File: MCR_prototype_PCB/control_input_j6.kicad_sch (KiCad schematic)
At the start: 34 parts, among them J6 Conn_01x10_Pin, U4 74AHC165

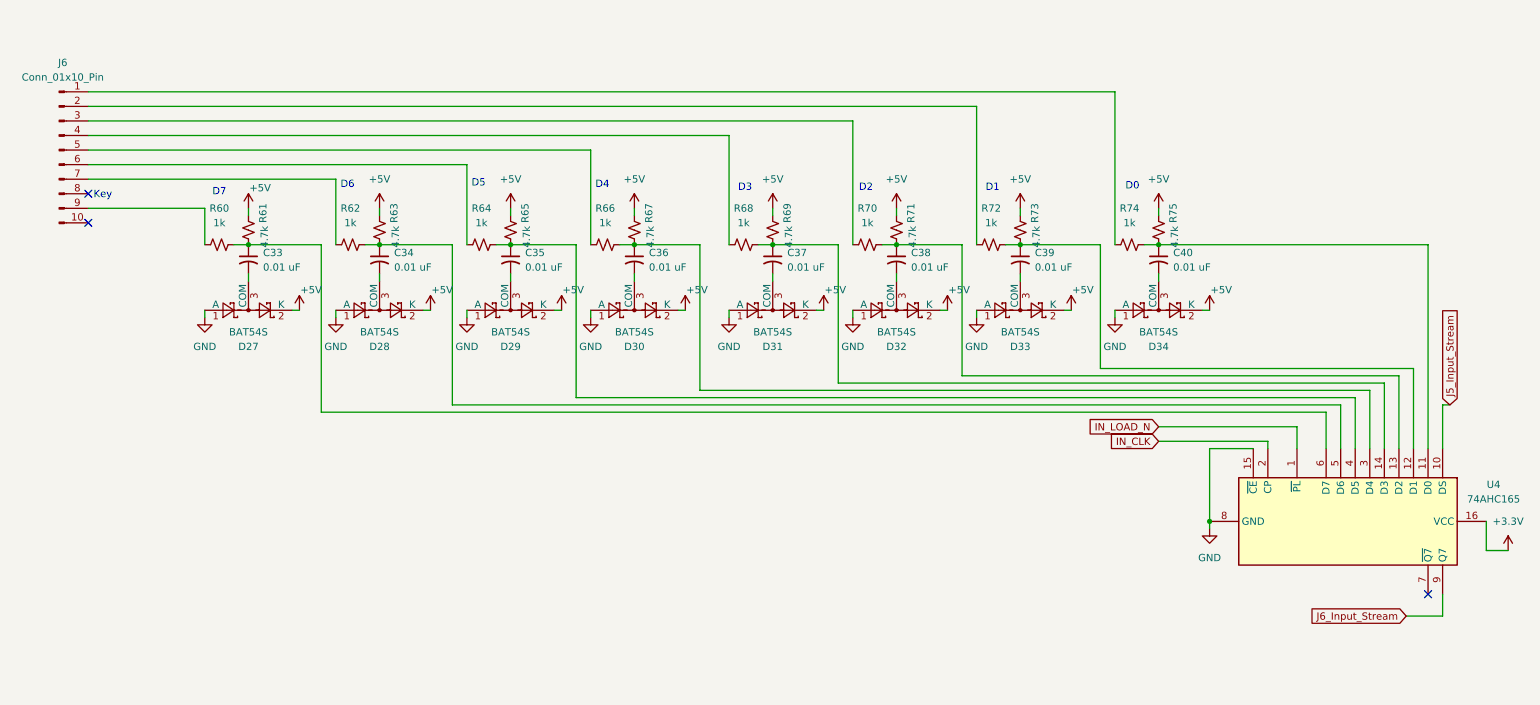
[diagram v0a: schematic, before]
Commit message: Updated 8/22/26
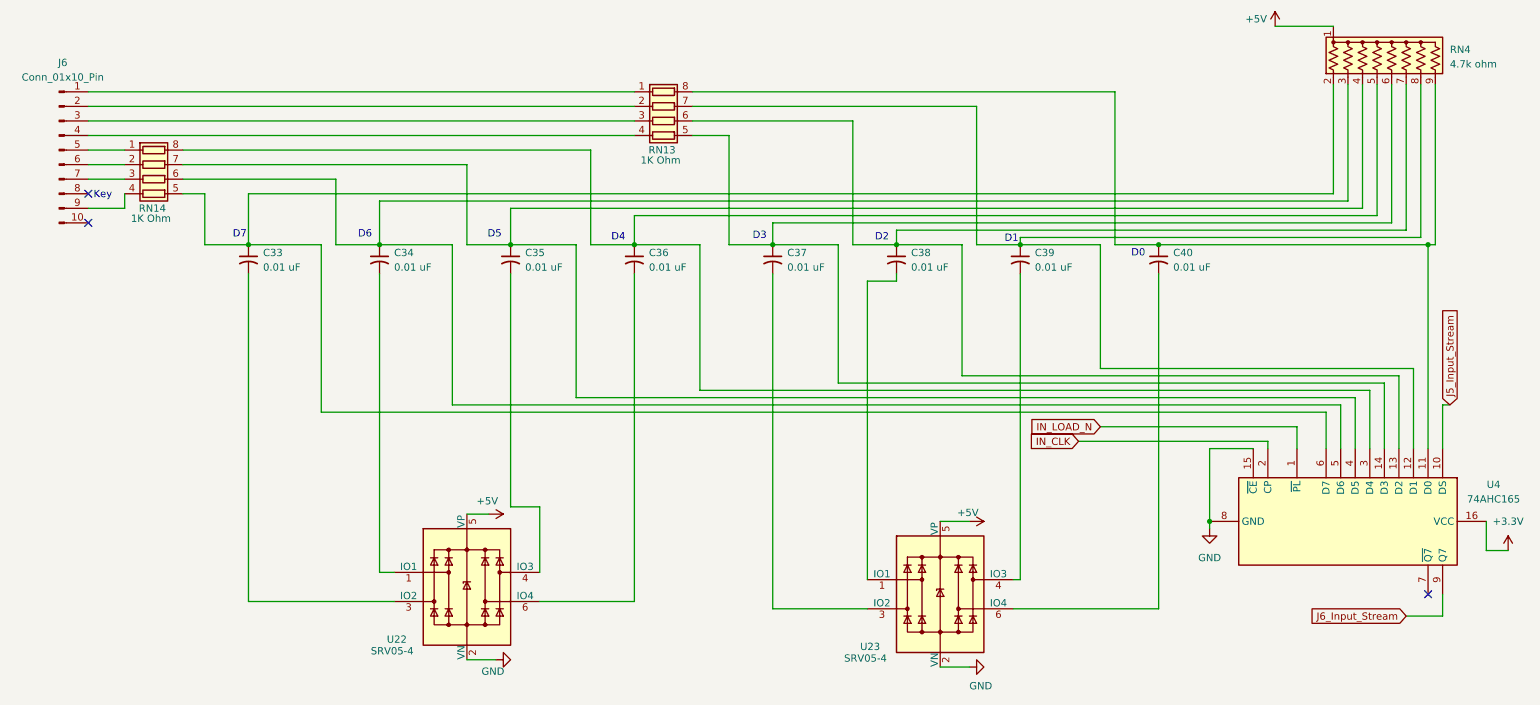
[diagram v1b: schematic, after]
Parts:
- removed D27, D28, D29, D30, D31, D32, D33, D34: BAT54S, Package_TO_SOT_SMD:SOT-23, symbol Diode:BAT54S
- removed R60, R62, R64, R66, R68, R70, R72, R74: 1k, Resistor_SMD:R_0805_2012Metric, symbol Device:R_Small_US
- removed R61, R63, R65, R67, R69, R71, R73, R75: 4.7k, Resistor_SMD:R_0805_2012Metric, symbol Device:R_Small_US
- added RN13, RN14: 1K Ohm, Resistor_SMD:R_Array_Convex_4x0603, symbol Device:R_Pack04
- added RN4: 4.7k ohm, Resistor_THT:R_Array_SIP9, symbol Device:R_Network08_US
- added U22, U23: SRV05-4, Package_TO_SOT_SMD:SOT-23-6, symbol Power_Protection:SRV05-4
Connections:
- net +5V: now also RN4.1 (common), U22.5 (VP), U23.5 (VP)
- net GND: now also U22.2 (VN), U23.2 (VN)
- net at C40.1, U4.11 (D0): now also RN13.8 (R1.2), RN4.9 (R8)
- net at C40.2: now also U23.6 (IO4)
- net at C37.1, U4.14 (D3): now also RN13.5 (R4.2), RN4.6 (R5)
- net at C39.1, U4.12 (D1): now also RN13.7 (R2.2), RN4.8 (R7)
- net at J6.1 (Pin_1): now also RN13.1 (R1.1)
- net at J6.2 (Pin_2): now also RN13.2 (R2.1)
- net at J6.3 (Pin_3): now also RN13.3 (R3.1)
- net at J6.4 (Pin_4): now also RN13.4 (R4.1)
- net at J6.5 (Pin_5): now also RN14.1 (R1.1)
- net at J6.6 (Pin_6): now also RN14.2 (R2.1)
- net at J6.7 (Pin_7): now also RN14.3 (R3.1)
- net at J6.9 (Pin_9): now also RN14.4 (R4.1)
- net at C33.1, U4.6 (D7): now also RN14.5 (R4.2), RN4.2 (R1)
- net at C34.2: now also U22.1 (IO1)
- net at C34.1, U4.5 (D6): now also RN14.6 (R3.2), RN4.3 (R2)
- net at C38.1, U4.13 (D2): now also RN13.6 (R3.2), RN4.7 (R6)
- net at C38.2: now also U23.1 (IO1)
- net at C39.2: now also U23.4 (IO3)
- net at C36.1, U4.3 (D4): now also RN14.8 (R1.2), RN4.5 (R4)
- net at C36.2: now also U22.6 (IO4)
- net at C35.1, U4.4 (D5): now also RN14.7 (R2.2), RN4.4 (R3)
- net at C33.2: now also U22.3 (IO2)
- net at C37.2: now also U23.3 (IO2)
- net at C35.2: now also U22.4 (IO3)
